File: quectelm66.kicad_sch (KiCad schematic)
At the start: 19 parts, among them J2 SIM8060-6-0-14-00-A, J5 U.FL-R-SMT-1(10), U10 M66

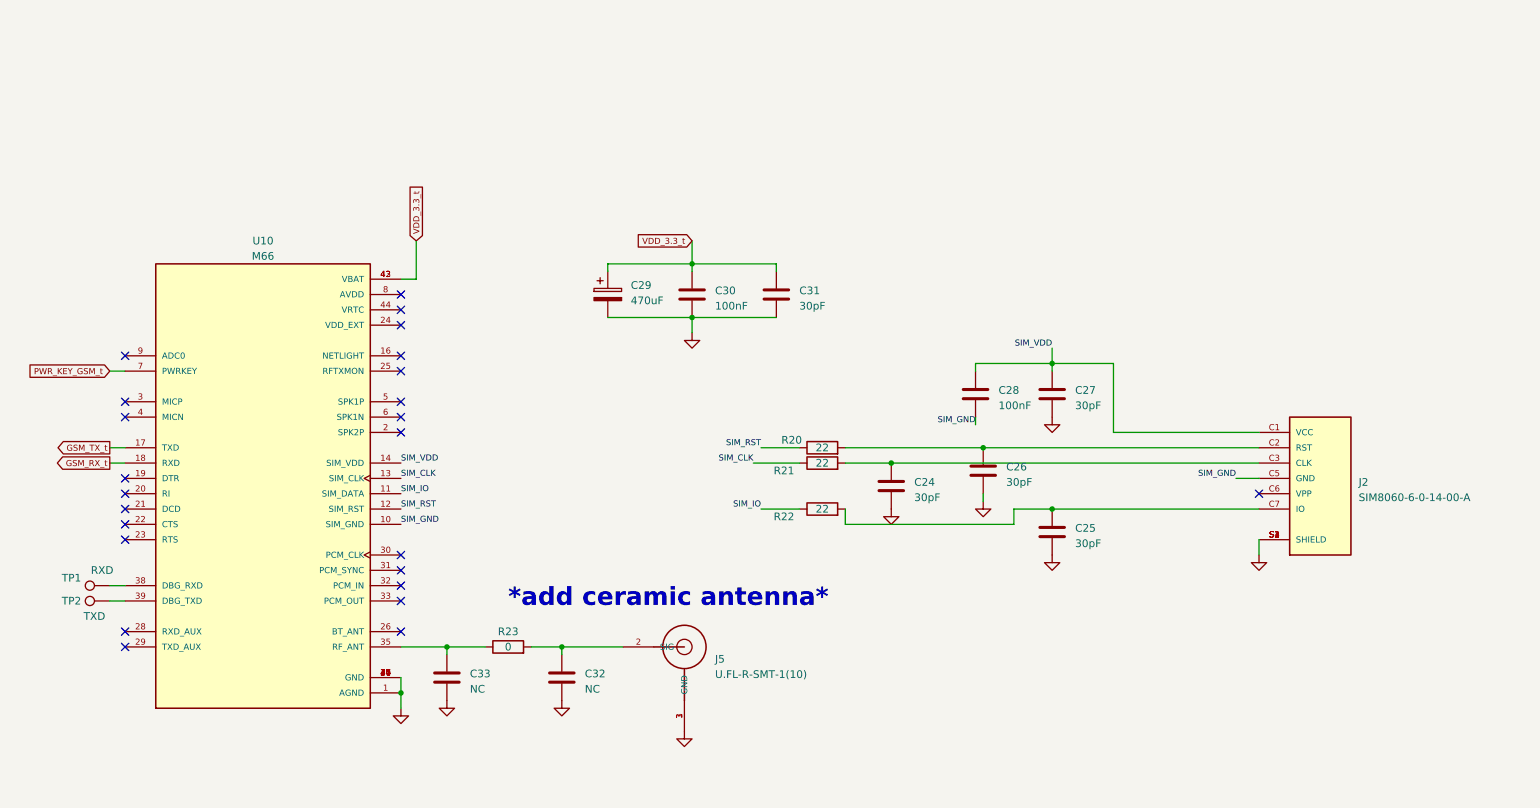
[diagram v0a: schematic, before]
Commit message: Final Design
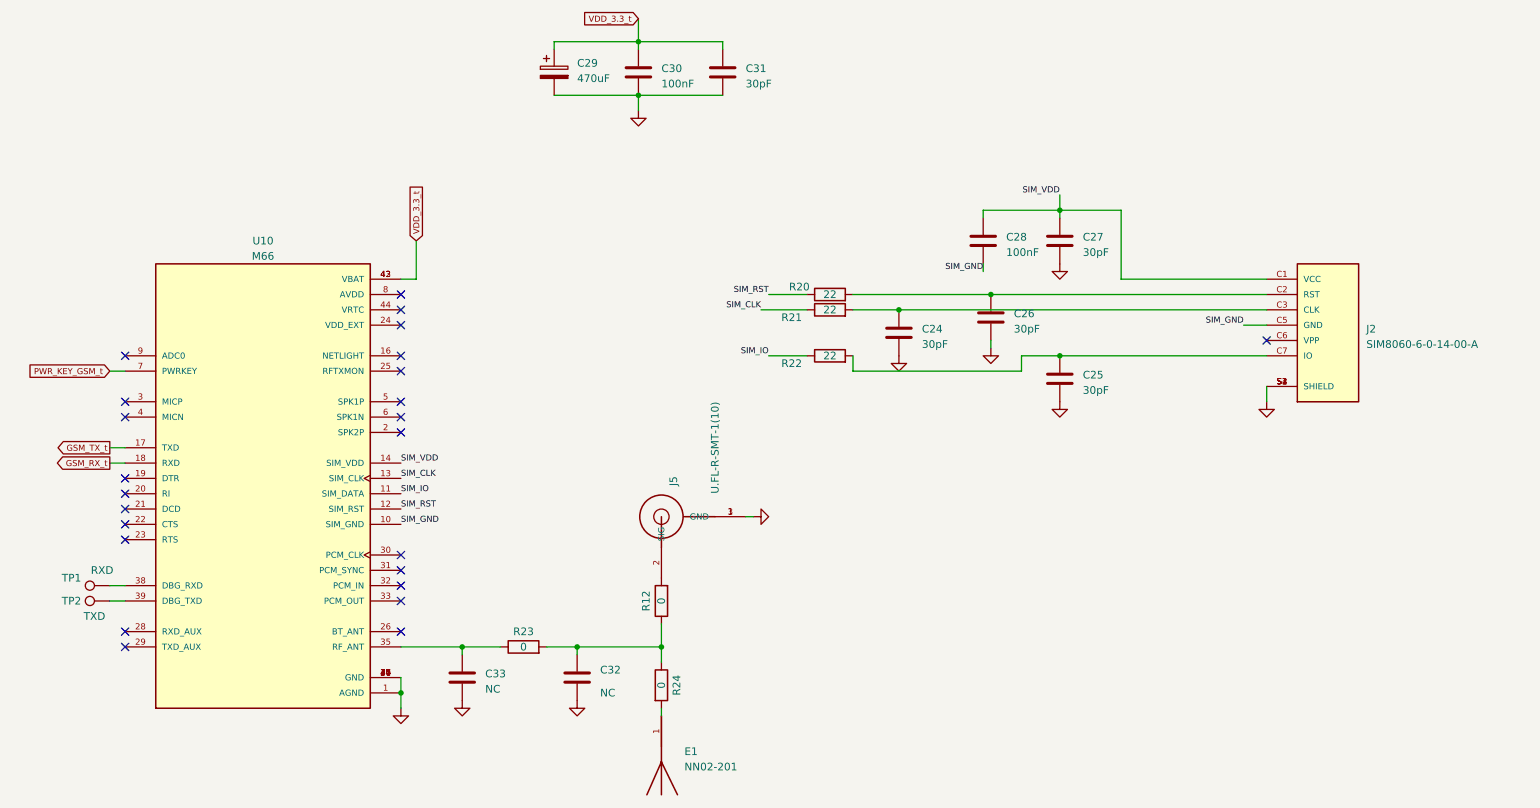
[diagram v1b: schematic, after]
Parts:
- added E1: NN02-201, NN02-201:XCVR_NN02-201, symbol NN02-201:NN02-201
- added R12, R24: 0, Resistor_SMD:R_0402_1005Metric_Pad0.72x0.64mm_HandSolder, symbol Device:R
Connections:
- net at C32.1, R23.2: now also R12.1, R24.1; no longer J5.2 (SIG)
- new net: J5.2 (SIG), R12.2
- new net: E1.1, R24.2
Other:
- note removed: "*add ceramic antenna*"
- moved on the sheet: C24, C25, C26, C27, C28, C29, C30, C31, C32, C33, J2, J5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
